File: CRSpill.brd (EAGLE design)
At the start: 70 x 22.2 mm, 23 parts, among them IC1 7805DT, IC2 BLUE_PILL, IC3 NCV7351D1E, J3 MA04-1, SW1 SWITCH_TACTILETOP, U1 STM32F103C8, U7 XC6206, X1 8P8C-LED

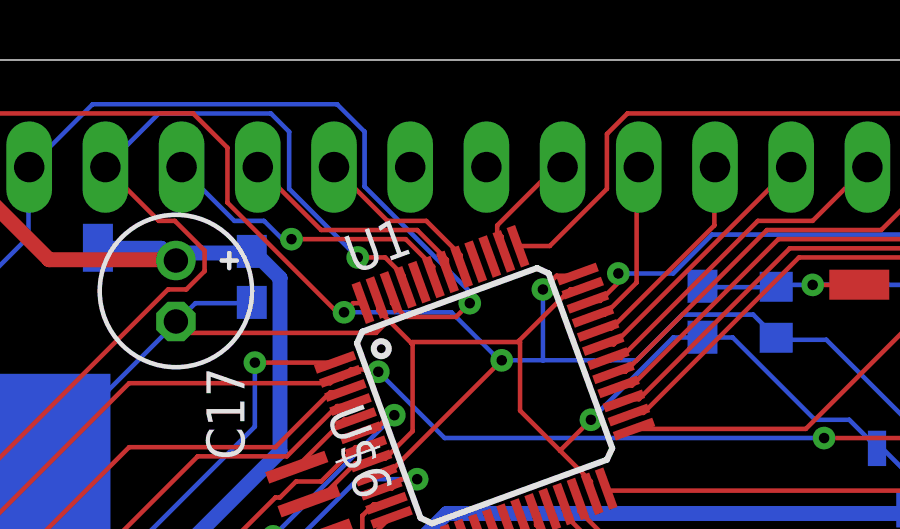
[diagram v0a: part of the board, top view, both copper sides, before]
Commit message: 未接続部を処理
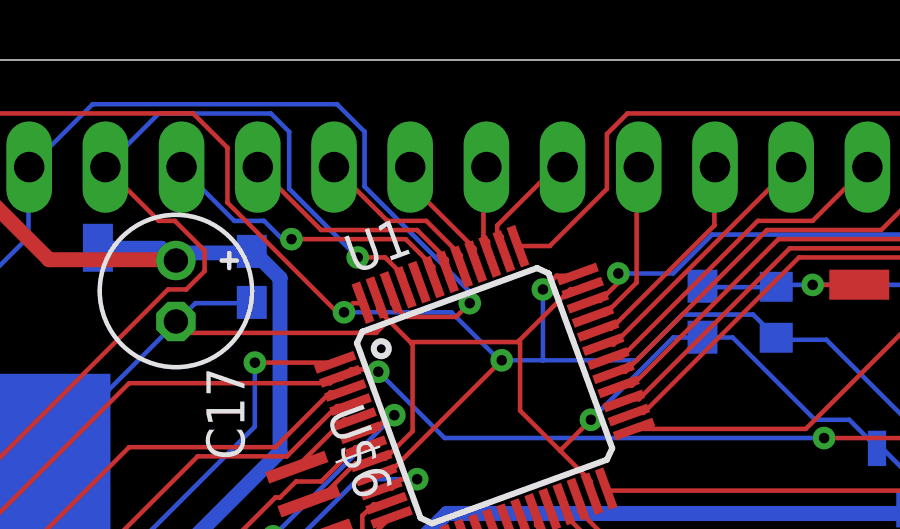
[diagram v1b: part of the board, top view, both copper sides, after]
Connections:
- removed net BP3: IC2.P$31
- removed net BP4: IC2.P$32
- net PB3: now also IC2.P$31
- net PB4: now also IC2.P$32
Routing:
- net PB4: track 0.00 -> 4.05 mm
- net PB3: track 0.00 -> 3.11 mm
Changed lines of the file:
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@@
 <signal name="PB3">
 <contactref element="U1" pad="39"/>
+<contactref element="IC2" pad="P$31"/>
+<wire x1="40.005" y1="16.6116" x2="40.005" y2="16.1544" width="0.1524" layer="1"/>
+<wire x1="39.8526" y1="16.764" x2="40.005" y2="16.6116" width="0.1524" layer="1"/>
+<wire x1="39.8526" y1="18.9738" x2="39.8526" y2="16.764" width="0.1524" layer="1"/>
+<wire x1="39.9288" y1="19.05" x2="39.8526" y2="18.9738" width="0.1524" layer="1"/>
+<wire x1="40.005" y1="16.1544" x2="40.063775" y2="16.1092125" width="0.1524" layer="1"/>
+<wire x1="39.9288" y1="19.05" x2="39.95" y2="19.09" width="0.1524" layer="1"/>
 </signal>
 <signal name="PB4">
 <contactref element="U1" pad="40"/>
+<contactref element="IC2" pad="P$32"/>
+<wire x1="39.5478" y1="16.383" x2="39.5478" y2="16.002" width="0.1524" layer="1"/>
+<wire x1="37.4142" y1="18.5166" x2="39.5478" y2="16.383" width="0.1524" layer="1"/>
+<wire x1="37.4142" y1="19.05" x2="37.4142" y2="18.5166" width="0.1524" layer="1"/>
+<wire x1="39.5478" y1="16.002" x2="39.593928125" y2="15.938203125" width="0.1524" layer="1"/>
+<wire x1="37.4142" y1="19.05" x2="37.41" y2="19.09" width="0.1524" layer="1"/>
 </signal>
 <signal name="PC15">
@@
 <wire x1="55.1688" y1="19.05" x2="55.19" y2="19.09" width="0.1524" layer="1"/>
 </signal>
-<signal name="BP4">
-<contactref element="IC2" pad="P$32"/>
-</signal>
-<signal name="BP3">
-<contactref element="IC2" pad="P$31"/>
-</signal>
 </signals>
